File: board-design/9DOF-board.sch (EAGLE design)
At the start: 13 parts

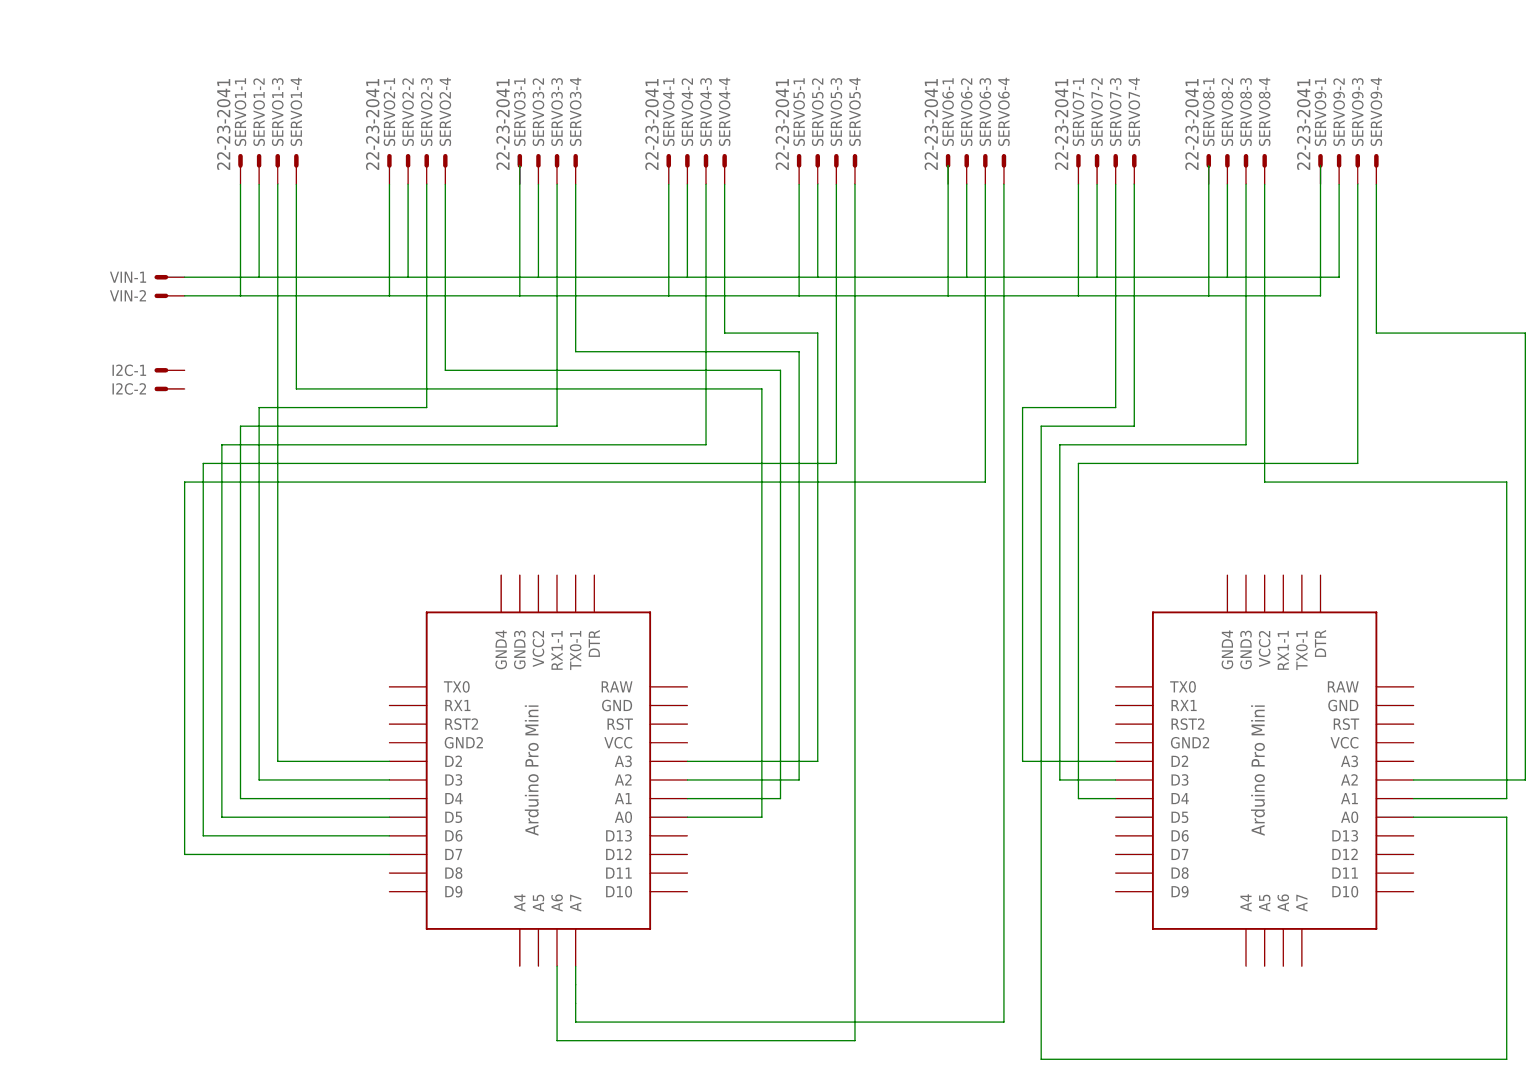
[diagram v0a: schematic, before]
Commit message: Add files via upload
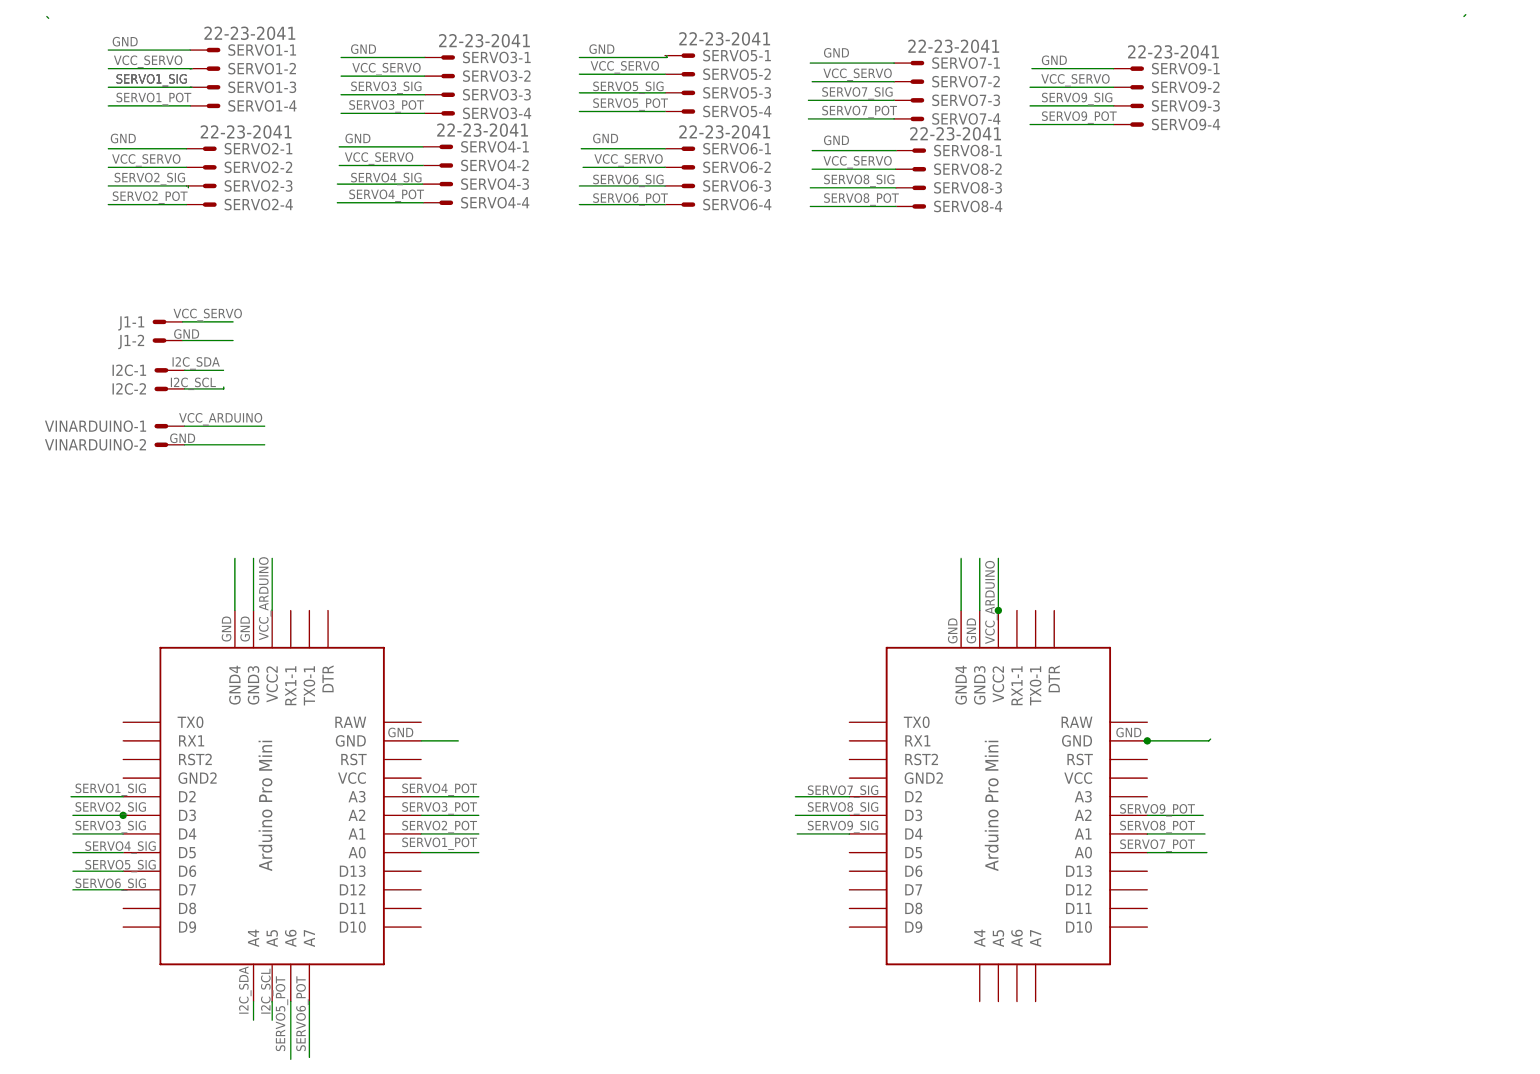
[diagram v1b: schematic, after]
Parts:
- removed VIN: 22-23-2021, con-molex:22-23-2021
- added J1, VINARDUINO: 22-23-2021, con-molex:22-23-2021
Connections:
- net N$1 renamed SERVO1_POT
- net N$10 renamed SERVO9_POT
- net N$11 renamed SERVO6_POT
- net N$12 renamed SERVO2_SIG
- net N$13 renamed SERVO7_POT
- net N$14 renamed SERVO3_SIG
- net N$15 renamed SERVO4_SIG
- net N$16 renamed SERVO5_SIG
- net N$17 renamed SERVO6_SIG
- net N$18 renamed SERVO8_POT
- net N$19 renamed SERVO9_SIG
- net N$2 renamed SERVO2_POT
- net N$20 renamed SERVO7_SIG
- net N$3 renamed SERVO3_POT
- net N$4 renamed SERVO4_POT
- net N$5 renamed SERVO1_SIG
- net N$7 renamed SERVO8_SIG
- net N$8 renamed SERVO5_POT
- removed net N$6: SERVO1-1.S, SERVO2-1.S, SERVO4-1.S, SERVO5-1.S, SERVO7-1.S, VIN-2.S
- removed net N$9: SERVO1-2.S, SERVO2-2.S, SERVO3-2.S, SERVO4-2.S, SERVO5-2.S, SERVO6-2.S, SERVO7-2.S, SERVO8-2.S, SERVO9-2.S, VIN-1.S
- new net GND: J1-2.S, SERVO1-1.S, SERVO2-1.S, SERVO3-1.S, SERVO4-1.S, SERVO6-1.S, SERVO7-1.S, SERVO8-1.S, SERVO9-1.S, U$1.GND, U$1.GND3, U$1.GND4, U$2.GND, U$2.GND3, U$2.GND4, VINARDUINO-2.S
- new net I2C_SCL: I2C-2.S, U$1.A5
- new net I2C_SDA: I2C-1.S, U$1.A4
- new net VCC_ARDUINO: U$1.VCC2, U$2.VCC2, VINARDUINO-1.S
- new net VCC_SERVO: J1-1.S, SERVO1-2.S, SERVO2-2.S, SERVO3-2.S, SERVO4-2.S, SERVO5-2.S, SERVO6-2.S, SERVO7-2.S, SERVO8-2.S, SERVO9-2.S
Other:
- moved on the sheet: SERVO1-1, SERVO1-2, SERVO1-3, SERVO1-4, SERVO2-1, SERVO2-2, SERVO2-3, SERVO2-4, SERVO3-1, SERVO3-2, SERVO3-3, SERVO3-4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
